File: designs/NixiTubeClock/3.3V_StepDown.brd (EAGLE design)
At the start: 31 x 34 mm, 10 parts, among them IC1 TPS62160DGKR, J1 S2B-PH-SM4, J2 S2B-PH-SM4

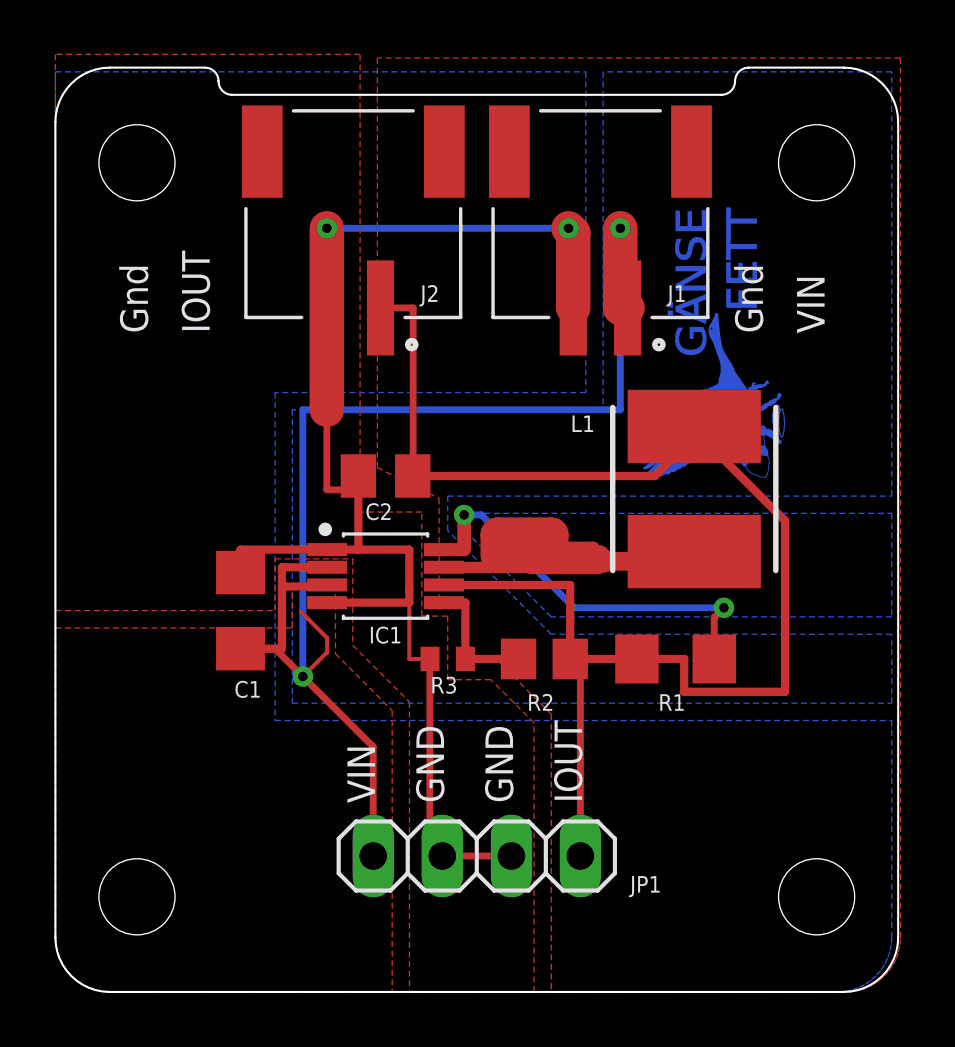
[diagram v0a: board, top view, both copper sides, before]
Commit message: started work on mainboard
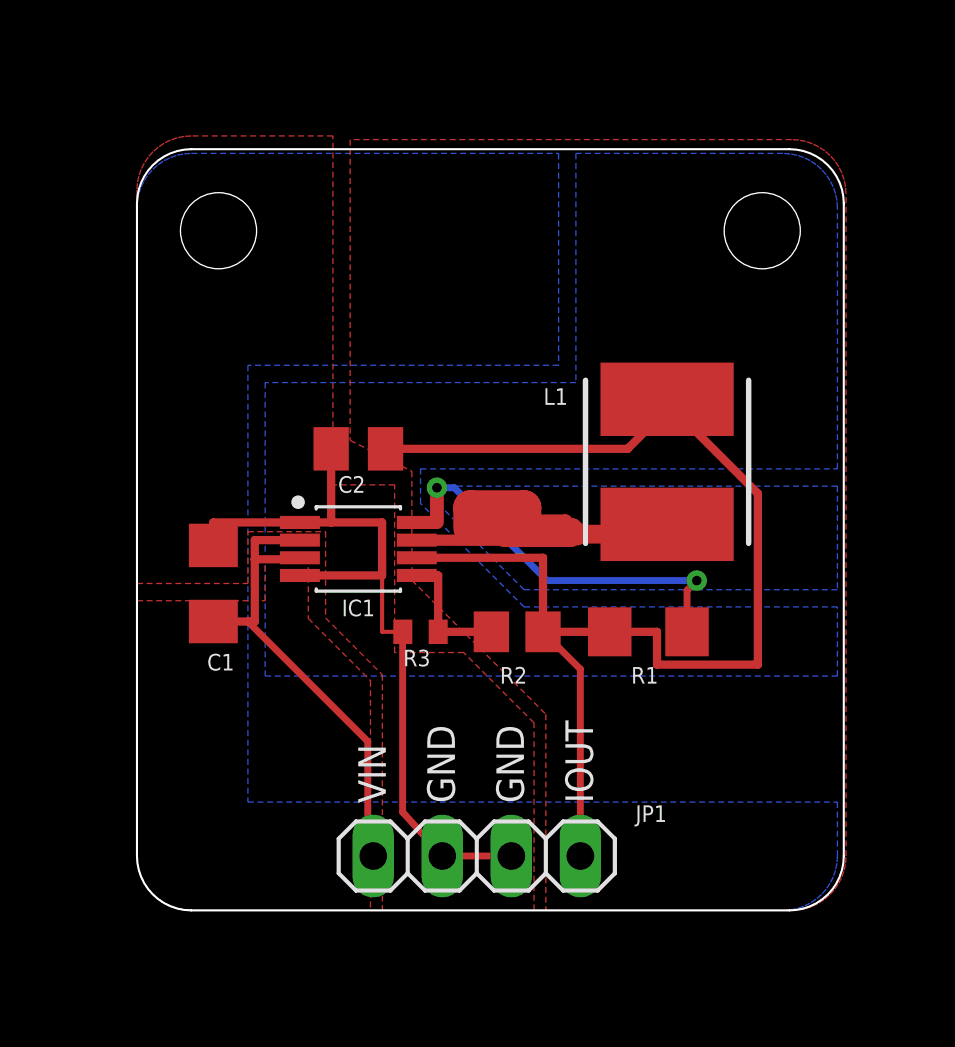
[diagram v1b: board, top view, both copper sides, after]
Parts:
- removed J1, J2: S2B-PH-SM4, CommonParts:JST_S2B-PH-SM4-TB(LF)(SN)
- moved C2 1.41 mm to (8.14, 17.0)
- moved C1 1.41 mm to (2.81, 12.0)
- moved IC1 1.41 mm to (8.14, 13.3)
- moved L1 1.41 mm to (19.5, 16.5)
- moved R1 1.41 mm to (18.8, 10.2)
- moved R2 1.41 mm to (14.0, 10.2)
- moved R3 1.41 mm to (10.4, 10.2)
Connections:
- net AGND: no longer J1.2, J2.2
- net IOUT: no longer J2.1
- net VIN: no longer J1.1
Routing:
- net VIN: track 52.6 -> 19.5 mm, vias 2 -> 0
- net AGND: track 55.0 -> 29.9 mm, vias 2 -> 0
- net IOUT: track 54.5 -> 48.6 mm
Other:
- board size 31 x 34 mm -> 26 x 28 mm
- board text removed: "Gnd"
